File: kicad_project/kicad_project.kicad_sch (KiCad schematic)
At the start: 28 parts, among them J1 USB_C_Receptacle_USB2.0_16P, Q1 DMG2302U, SW1 SW_Push, U1 STM32F031F6Px, U2 MCP73831-2-MC, U3 MCP4011-xxxxMS, U4 FT232RL, U5 LMZM23601

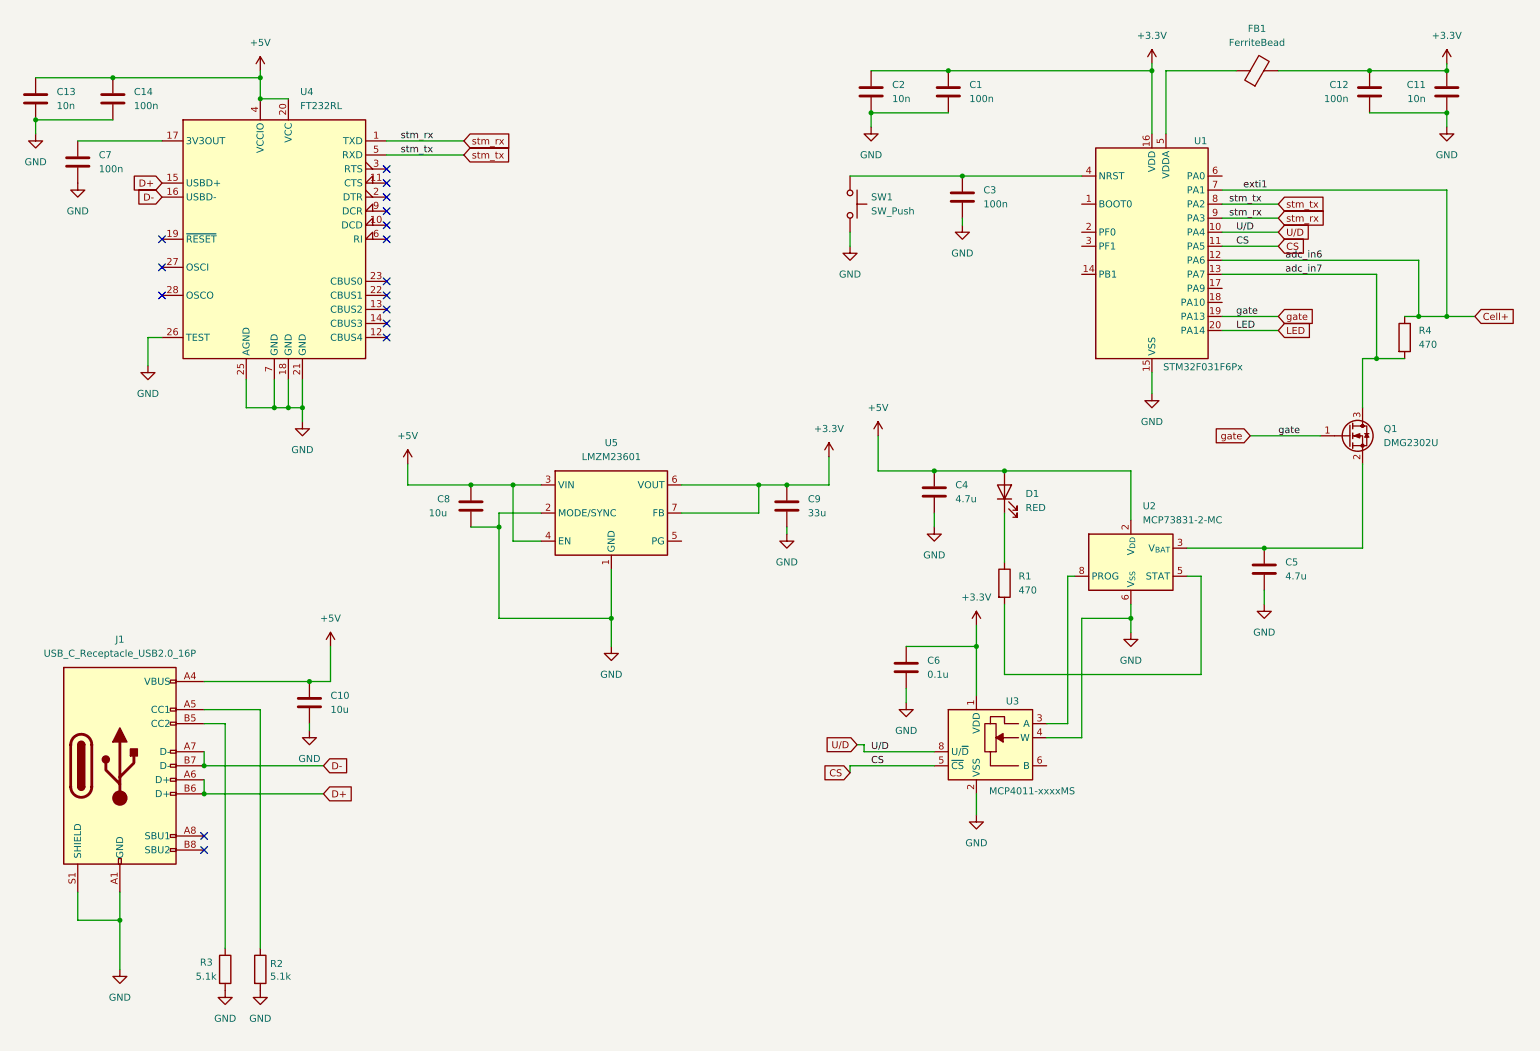
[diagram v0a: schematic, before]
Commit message: seg done
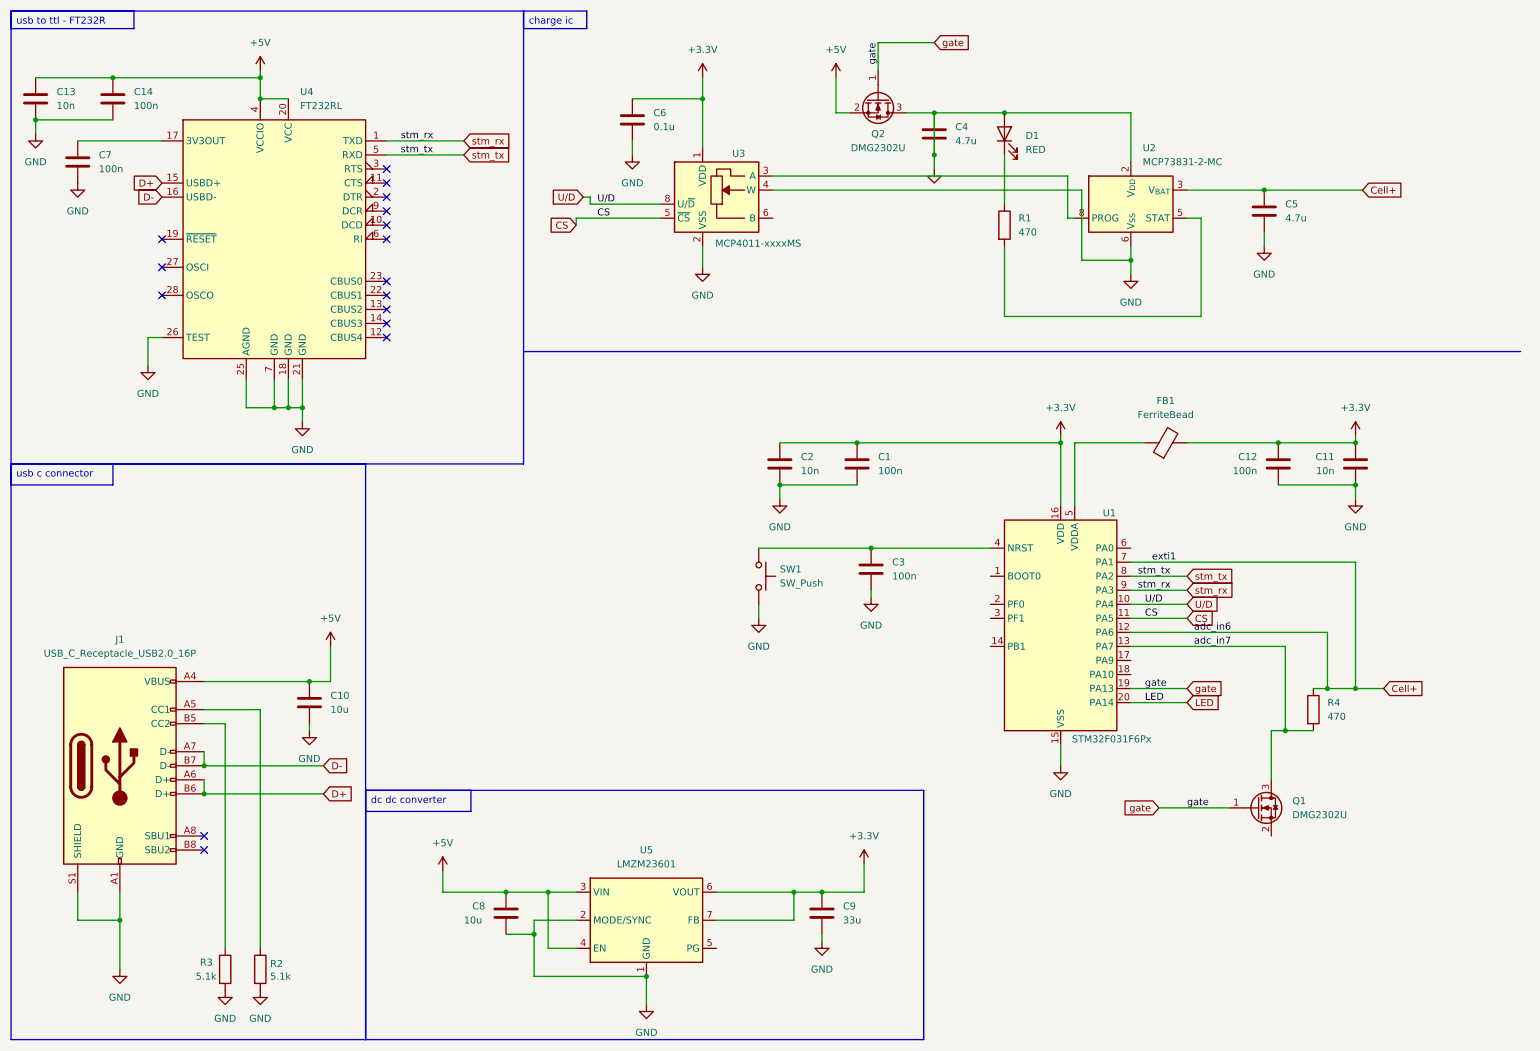
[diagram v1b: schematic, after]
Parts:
- added Q2: DMG2302U, Package_TO_SOT_SMD:SOT-23, symbol Transistor_FET:DMG2302U
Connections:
- net +5V: now also Q2.2 (S); no longer C4.1, D1.2 (A), U2.1 (V_{DD}), U2.2 (V_{DD})
- net Cell+: now also C5.1, U2.3 (V_{BAT}), U2.4 (V_{BAT})
- net GND: now also C4.1, D1.2 (A), U2.1 (V_{DD}), U2.2 (V_{DD}), Q2.3 (D)
- net gate: now also Q2.1 (G)
- now unconnected: Q1.2 (S)
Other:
- moved on the sheet: C1, C11, C12, C2, C3, C4, C5, C6, C8, C9, D1, FB1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
